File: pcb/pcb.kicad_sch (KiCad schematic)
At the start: 93 parts, among them J1 N!N, J10 Conn_01x12_Socket, J11 Conn_01x12_Socket, J12 Conn_01x02_Socket, J2 Conn_01x12_Socket, J3 Conn_01x12_Socket, J4 Conn_01x12_Socket, J5 Conn_01x12_Socket, J6 Display_nice-view, J7 Conn_01x02_Socket, J8 Conn_01x12_Socket, J9 Conn_01x12_Socket, SW1 Switch, SW10 Switch, SW11 Switch, SW12 Switch, SW13 Switch, SW14 Switch, SW15 Switch, SW16 Switch, SW17 Switch, SW18 Switch, SW19 Switch, SW2 Switch, SW20 Switch, SW21 Switch, SW22 Switch, SW23 Switch, SW24 Switch, SW25 Switch, SW26 Switch, SW27 Switch, SW28 Switch, SW29 Switch, SW3 Switch, SW30 Switch, SW31 Switch, SW32 Switch, SW33 Switch, SW34 Switch, SW35 Switch, SW36 Switch, SW37 SW_Push, SW38 RotaryEncoder_Switch, SW4 Switch, SW5 Switch, SW6 Switch, SW7 Switch, SW8 Switch, SW9 Switch

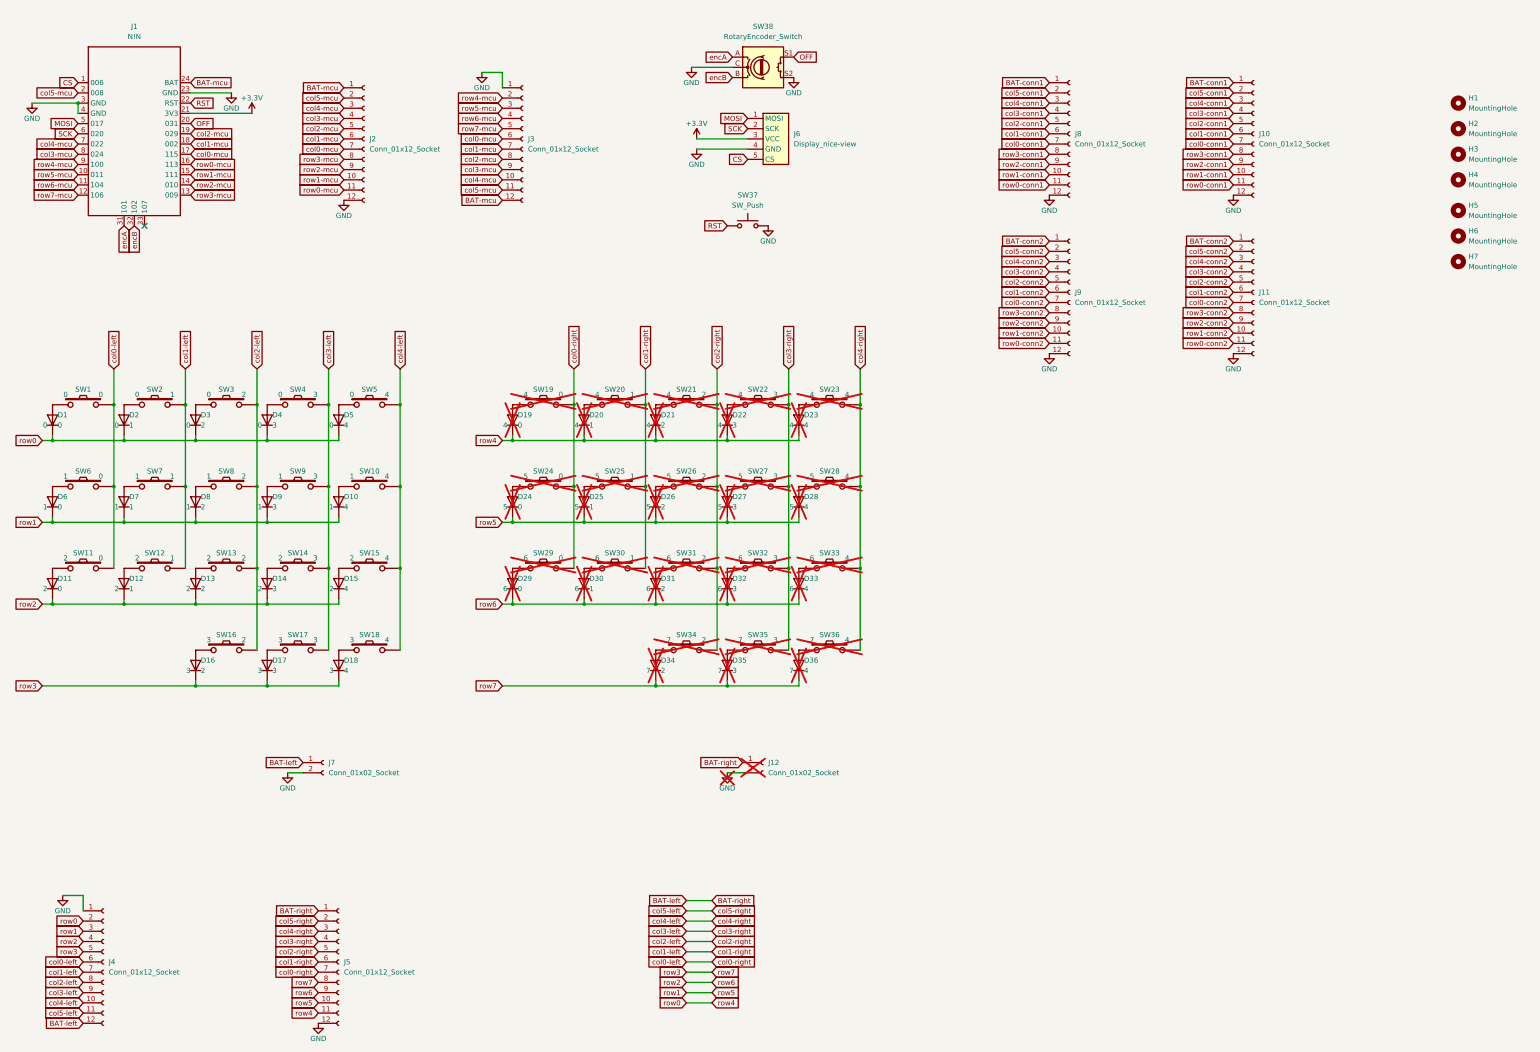
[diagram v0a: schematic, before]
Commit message: second draft
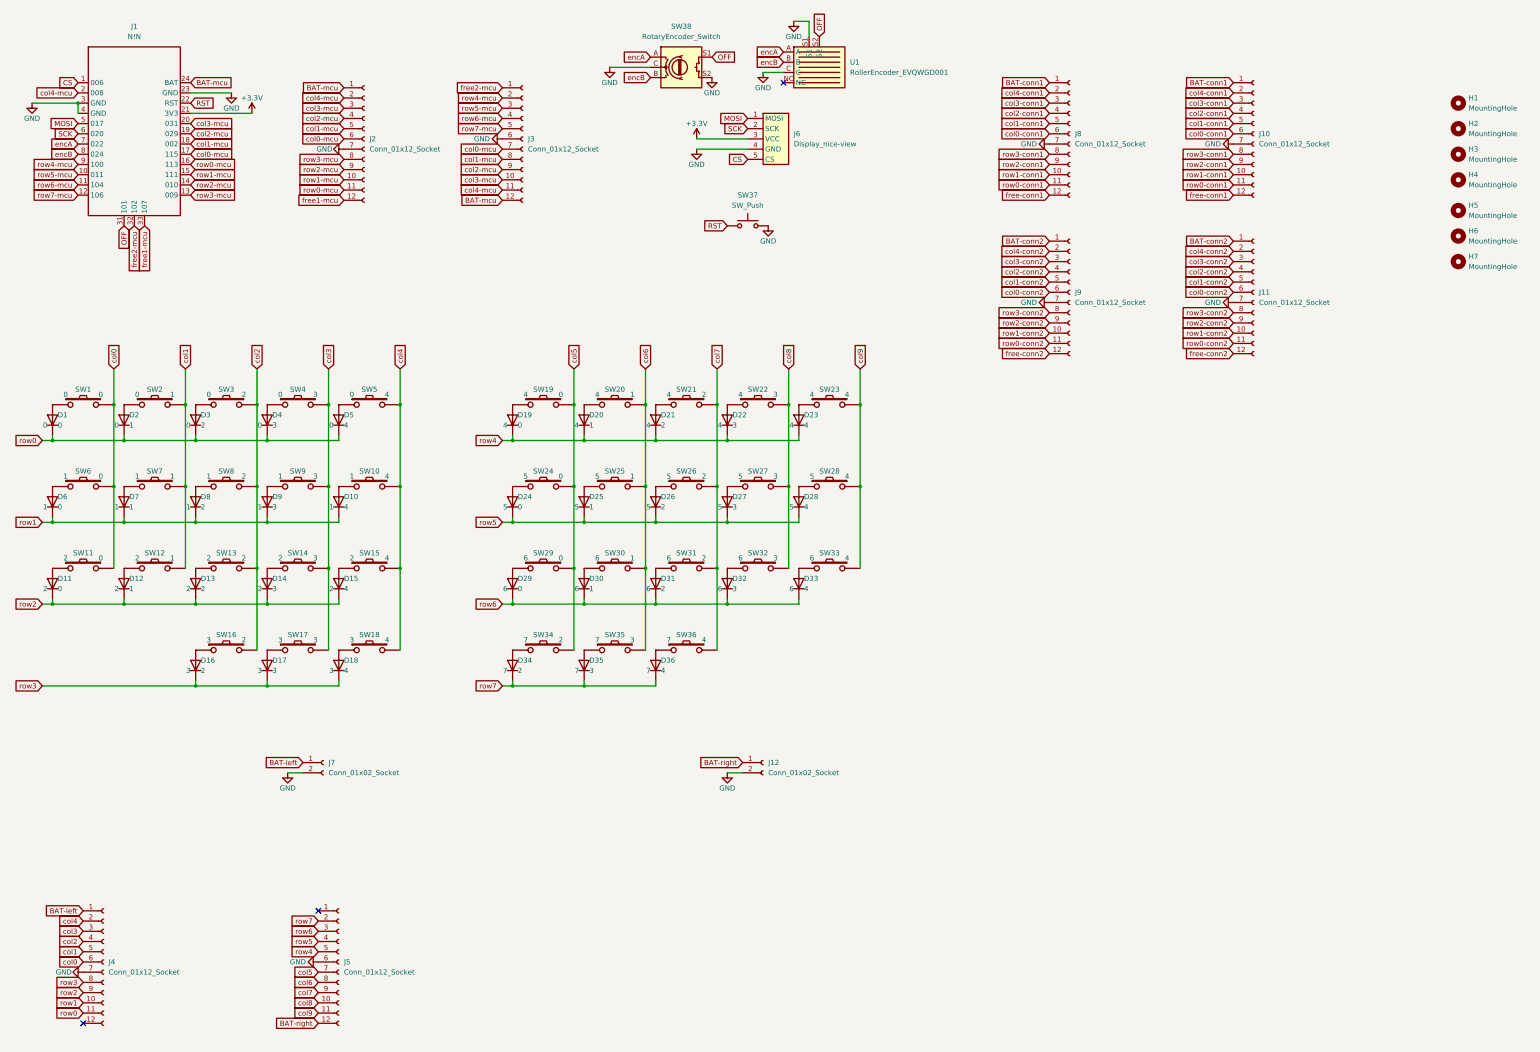
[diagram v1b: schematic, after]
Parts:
- added U1: RollerEncoder_EVQWGD001, zzkeeb:RotaryEncoder_EVQWGD001, symbol zzkeeb:RollerEncoder_EVQWGD001
- D1, D10, D11, D12, D13, D14, D15, D16, D17, D18, D2, D3, D4, D5, D6, D7, D8, D9: footprint zzkeeb:Diode_1N4148-SOD123-no-label-reversible -> zzkeeb:Diode_1N4148-SOD123
- D19, D20, D21, D22, D23, D24, D25, D26, D27, D28, D29, D30, D31, D32, D33, D34, D35, D36: footprint zzkeeb:Diode_1N4148-SOD123-no-label -> zzkeeb:Diode_1N4148-SOD123; now fitted
- H1, H2, H3, H4, H5, H6, H7: footprint zzkeeb:Hole_M2-TH -> zzkeeb:Hole_M2-solder-nut-2.5
- J12, SW19, SW20, SW21, SW22, SW23, SW24, SW25, SW26, SW27, SW28, SW29, SW30, SW31, SW32, SW33, SW34, SW35, SW36: now fitted
- SW1, SW10, SW11, SW12, SW13, SW14, SW15, SW16, SW17, SW18, SW2, SW3, SW4, SW5, SW6, SW7, SW8, SW9: footprint zzkeeb:Switch_KS-miny-reversible-hotswap-south -> zzkeeb:Switch_MXKS-miny-hotswap-south-ks3d
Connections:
- net col5-conn1 is gone; now on net col4-conn1: J10.2 (Pin_2), J8.2 (Pin_2)
- net col5-conn2 is gone; now on net col4-conn2: J11.2 (Pin_2), J9.2 (Pin_2)
- net col5-mcu is gone; now on net col4-mcu: J1.2 (008), J2.2 (Pin_2), J3.11 (Pin_11)
- net BAT-left: now also J4.1 (Pin_1); no longer J12.1 (Pin_1), J4.12 (Pin_12), J5.1 (Pin_1)
- net GND: now also J10.7 (Pin_7), J11.7 (Pin_7), J2.7 (Pin_7), J3.6 (Pin_6), J4.7 (Pin_7), J5.6 (Pin_6), J8.7 (Pin_7), J9.7 (Pin_7), U1.C, U1.S1; no longer J10.12 (Pin_12), J11.12 (Pin_12), J2.12 (Pin_12), J3.1 (Pin_1), J4.1 (Pin_1), J5.12 (Pin_12), J8.12 (Pin_12), J9.12 (Pin_12)
- net OFF: now also J1.31 (101), U1.S2; no longer J1.20 (031)
- net col0-conn1: now also J10.6 (Pin_6), J8.6 (Pin_6); no longer J10.7 (Pin_7), J8.7 (Pin_7)
- net col0-conn2: now also J11.6 (Pin_6), J9.6 (Pin_6); no longer J11.7 (Pin_7), J9.7 (Pin_7)
- net col0-mcu: now also J2.6 (Pin_6), J3.7 (Pin_7); no longer J2.7 (Pin_7), J3.6 (Pin_6)
- net col1-conn1: now also J10.5 (Pin_5), J8.5 (Pin_5); no longer J10.6 (Pin_6), J8.6 (Pin_6)
- net col1-conn2: now also J11.5 (Pin_5), J9.5 (Pin_5); no longer J11.6 (Pin_6), J9.6 (Pin_6)
- net col1-mcu: now also J2.5 (Pin_5), J3.8 (Pin_8); no longer J2.6 (Pin_6), J3.7 (Pin_7)
- net col2-conn1: now also J10.4 (Pin_4), J8.4 (Pin_4); no longer J10.5 (Pin_5), J8.5 (Pin_5)
- net col2-conn2: now also J11.4 (Pin_4), J9.4 (Pin_4); no longer J11.5 (Pin_5), J9.5 (Pin_5)
- net col2-mcu: now also J2.4 (Pin_4), J3.9 (Pin_9); no longer J2.5 (Pin_5), J3.8 (Pin_8)
- net col3-conn1: now also J10.3 (Pin_3), J8.3 (Pin_3); no longer J10.4 (Pin_4), J8.4 (Pin_4)
- net col3-conn2: now also J11.3 (Pin_3), J9.3 (Pin_3); no longer J11.4 (Pin_4), J9.4 (Pin_4)
- net col3-mcu: now also J1.20 (031), J2.3 (Pin_3), J3.10 (Pin_10); no longer J1.8 (024), J2.4 (Pin_4), J3.9 (Pin_9)
- net col4-conn1: no longer J10.3 (Pin_3), J8.3 (Pin_3)
- net col4-conn2: no longer J11.3 (Pin_3), J9.3 (Pin_3)
- net col4-mcu: no longer J1.7 (022), J2.3 (Pin_3), J3.10 (Pin_10)
- net encA: now also J1.7 (022), U1.A; no longer J1.31 (101)
- net encB: now also J1.8 (024), U1.B; no longer J1.32 (102)
- net row0: now also J4.11 (Pin_11); no longer D19.1 (K), D20.1 (K), D21.1 (K), D22.1 (K), D23.1 (K), J4.2 (Pin_2), J5.11 (Pin_11)
- net row1: now also J4.10 (Pin_10); no longer D24.1 (K), D25.1 (K), D26.1 (K), D27.1 (K), D28.1 (K), J4.3 (Pin_3), J5.10 (Pin_10)
- net row2: now also J4.9 (Pin_9); no longer D29.1 (K), D30.1 (K), D31.1 (K), D32.1 (K), D33.1 (K), J4.4 (Pin_4), J5.9 (Pin_9)
- net row3: now also J4.8 (Pin_8); no longer D34.1 (K), D35.1 (K), D36.1 (K), J4.5 (Pin_5), J5.8 (Pin_8)
- net free1-mcu: now reaches J1.33 (107)
- net free1-mcu: now also J2.12 (Pin_12)
- net col0-left renamed col0
- net col0: no longer J5.7 (Pin_7), SW19.2, SW24.2, SW29.2
- removed net col1-left: J4.7 (Pin_7), J5.6 (Pin_6), SW12.2, SW2.2, SW20.2, SW25.2, SW30.2, SW7.2
- removed net col2-left: J4.8 (Pin_8), J5.5 (Pin_5), SW13.2, SW16.2, SW21.2, SW26.2, SW3.2, SW31.2, SW34.2, SW8.2
- removed net col3-left: J4.9 (Pin_9), J5.4 (Pin_4), SW14.2, SW17.2, SW22.2, SW27.2, SW32.2, SW35.2, SW4.2, SW9.2
- removed net col4-left: J4.10 (Pin_10), J5.3 (Pin_3), SW10.2, SW15.2, SW18.2, SW23.2, SW28.2, SW33.2, SW36.2, SW5.2
- net col5-left renamed row7
- net row7: now also D34.1 (K), D35.1 (K), D36.1 (K); no longer J4.11 (Pin_11)
- new net BAT-right: J12.1 (Pin_1), J5.12 (Pin_12)
- new net col1: J4.5 (Pin_5), SW12.2, SW2.2, SW7.2
- new net col2: J4.4 (Pin_4), SW13.2, SW16.2, SW3.2, SW8.2
- new net col3: J4.3 (Pin_3), SW14.2, SW17.2, SW4.2, SW9.2
- new net col4: J4.2 (Pin_2), SW10.2, SW15.2, SW18.2, SW5.2
- new net col5: J5.7 (Pin_7), SW19.2, SW24.2, SW29.2, SW34.2
- new net col6: J5.8 (Pin_8), SW20.2, SW25.2, SW30.2, SW35.2
- new net col7: J5.9 (Pin_9), SW21.2, SW26.2, SW31.2, SW36.2
- new net col8: J5.10 (Pin_10), SW22.2, SW27.2, SW32.2
- new net col9: J5.11 (Pin_11), SW23.2, SW28.2, SW33.2
- new net free-conn1: J10.12 (Pin_12), J8.12 (Pin_12)
- new net free-conn2: J11.12 (Pin_12), J9.12 (Pin_12)
- new net free2-mcu: J1.32 (102), J3.1 (Pin_1)
- new net row4: D19.1 (K), D20.1 (K), D21.1 (K), D22.1 (K), D23.1 (K), J5.5 (Pin_5)
- new net row5: D24.1 (K), D25.1 (K), D26.1 (K), D27.1 (K), D28.1 (K), J5.4 (Pin_4)
- new net row6: D29.1 (K), D30.1 (K), D31.1 (K), D32.1 (K), D33.1 (K), J5.3 (Pin_3)
- no-connect marks 1 -> 3
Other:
- moved on the sheet: SW38
